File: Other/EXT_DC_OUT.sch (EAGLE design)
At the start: 19 parts, among them IC1 TINY45, Q1 IRLU3410, Q2 IRLU3410, Q3 IRLU3410, X2 PW1

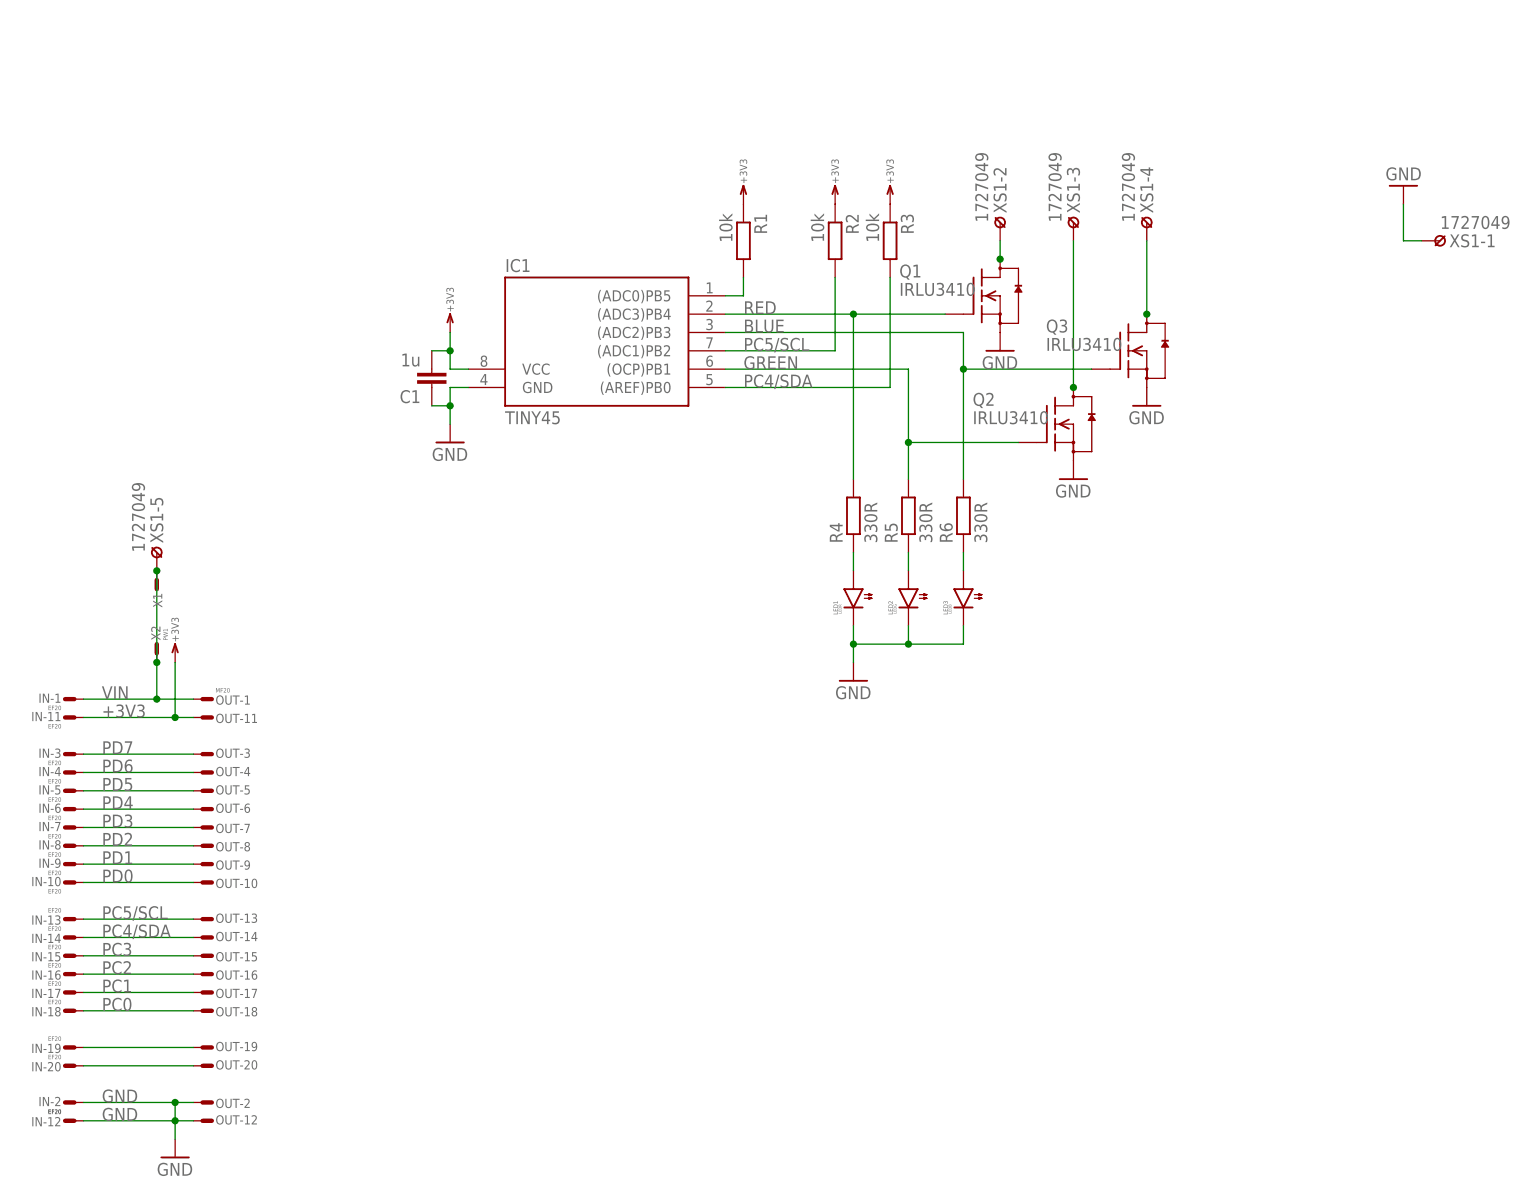
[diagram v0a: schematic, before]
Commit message: Added ...
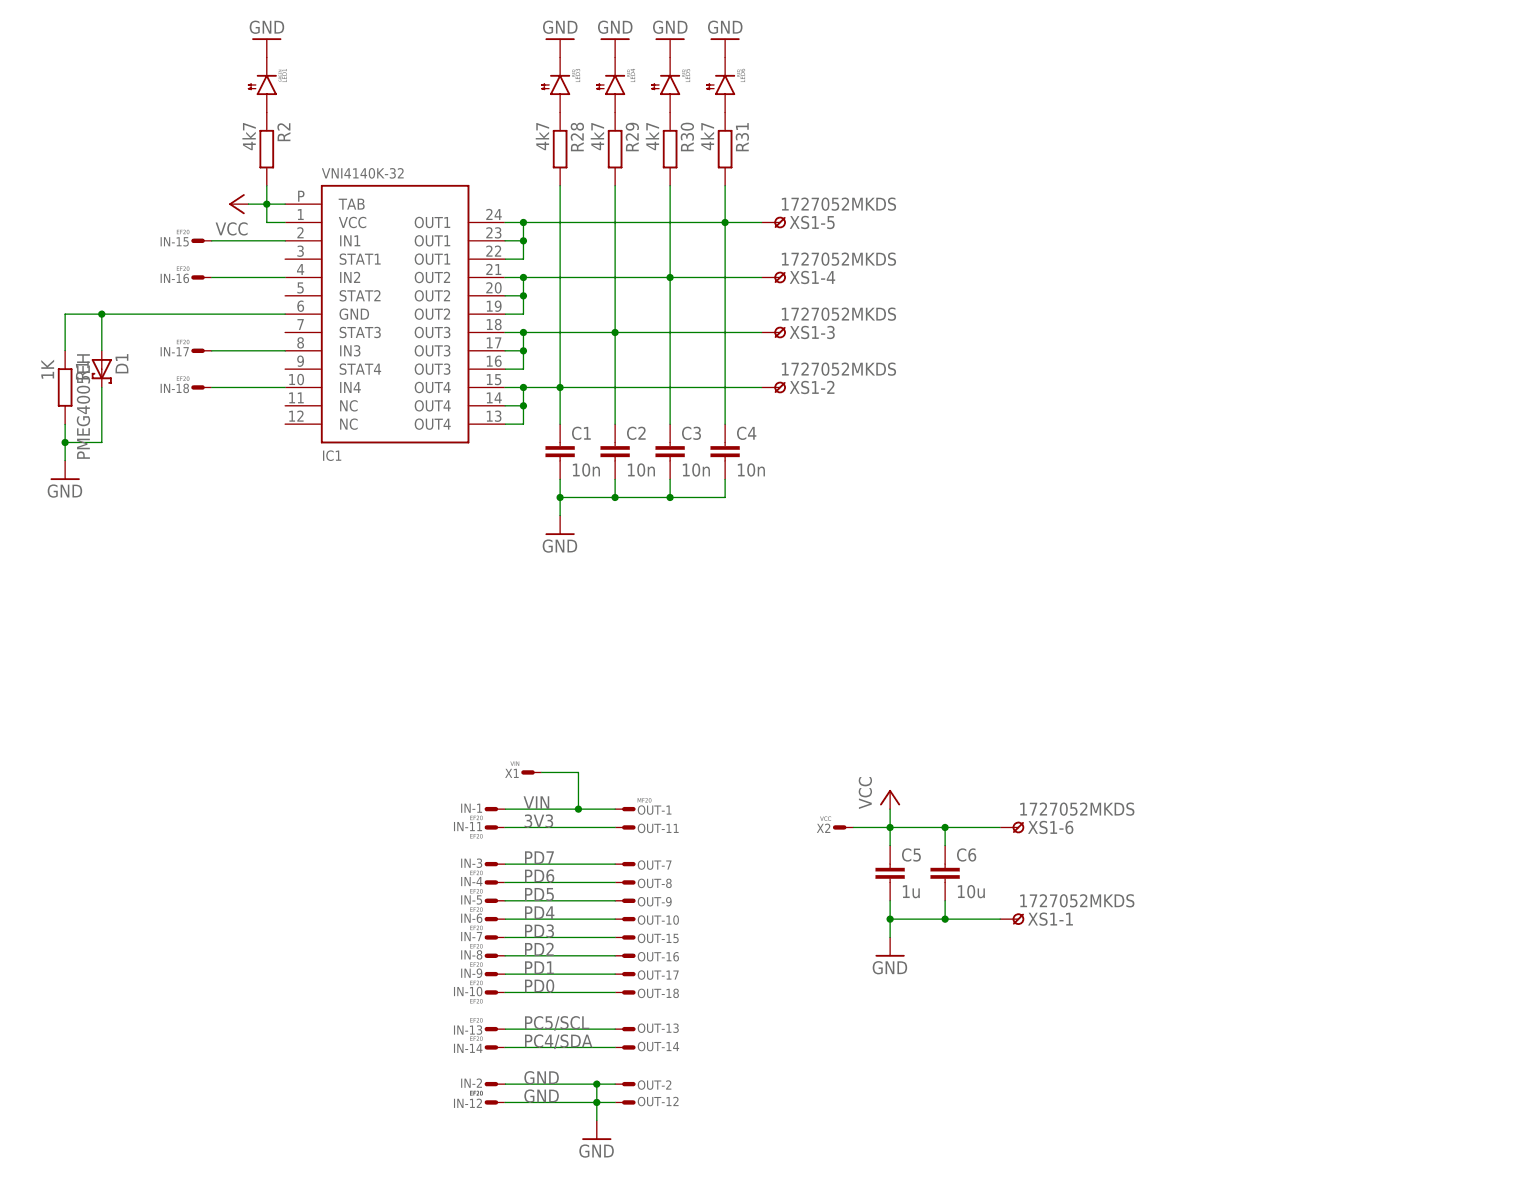
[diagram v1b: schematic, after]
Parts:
- removed LED2: LEDG, Optic:LED1206
- removed Q1, Q2, Q3: IRLU3410, Transistor:FET-ND251
- removed R3: 10k, RCL:R0603
- removed R4, R5, R6: 330R, RCL:R0603
- added C2, C3, C4: 10n, RCL:C1206
- added C5: 1u, RCL:C1206
- added C6: 10u, RCL:CC1210
- added D1: PMEG4005EH, Diode:D-SCHOTKY123
- added LED4, LED5, LED6: RED, Optic:LED1206
- added R28, R29, R30, R31: 4k7, RCL:R1206
- C1: value 1u -> 10n; device RCL:C0603 -> RCL:C1206
- IC1: value TINY45 -> VNI4140K-32; device atmel:TINY15LS -> ICs:VNI4140
- LED1: value LEDR -> GREEN
- LED3: value LEDB -> RED
- R1: value 10k -> 1K; device RCL:R0603 -> RCL:R1206
- R2: value 10k -> 4k7; device RCL:R0603 -> RCL:R1206
- X1: value (none) -> VIN
- X2: value PW1 -> VCC
- XS1: value 1727049 -> 1727052MKDS; device Conn:1727049 -> Conn:1727052MKDS
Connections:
- removed net +3V3: C1.2, IC1.VCC, IN-11.S, OUT-11.S, R1.1, R2.1, R3.1
- removed net BLUE: IC1.(ADC2)PB3, Q3.G, R6.2
- removed net GREEN: IC1.(OCP)PB1, Q2.G, R5.2
- removed net PC0: IN-18.S, OUT-18.S
- removed net PC1: IN-17.S, OUT-17.S
- removed net PC2: IN-16.S, OUT-16.S
- removed net PC3: IN-15.S, OUT-15.S
- removed net RED: IC1.(ADC3)PB4, Q1.G, R4.2
- removed net RST: IC1.(ADC0)PB5, R1.2
- new net 3V3: IN-11.S, OUT-11.S
- new net N$10: LED1.A, R2.1
- new net N$12: LED3.A, R28.1
- new net N$14: LED4.A, R29.1
- new net N$16: LED5.A, R30.1
- new net N$18: LED6.A, R31.1
- new net N$2: IC1.IN2, IN-16.S
- new net VCC: C5.1, C6.1, IC1.TAB, IC1.VCC, R2.2, X2.S, XS1-6.K
- net GND: now also C1.2, C2.2, C3.2, C4.2, C5.2, C6.2, D1.C, LED4.C, LED5.C, LED6.C, R1.2; no longer C1.1, IC1.GND, LED2.C, Q1.S, Q2.S, Q3.S
- net N$1: now also IC1.IN1, IN-15.S; no longer IN-20.S, OUT-20.S
- net N$3: now also IC1.IN3, IN-17.S; no longer IN-19.S, OUT-19.S
- net N$4: now also IC1.IN4, IN-18.S; no longer LED1.A, R4.1
- net N$5: now also C4.1, IC1.OUT1@22, IC1.OUT1@23, IC1.OUT1@24, R31.2, XS1-5.K; no longer LED2.A, R5.1
- net N$6: now also C3.1, IC1.OUT2@19, IC1.OUT2@20, IC1.OUT2@21, R30.2, XS1-4.K; no longer Q1.D, XS1-2.K
- net N$7: now also C2.1, IC1.OUT3@16, IC1.OUT3@17, IC1.OUT3@18, R29.2; no longer Q2.D
- net N$8: now also C1.1, IC1.OUT4@13, IC1.OUT4@14, IC1.OUT4@15, R28.2, XS1-2.K; no longer Q3.D, XS1-4.K
- net N$9: now also D1.A, IC1.GND, R1.1; no longer LED3.A, R6.1
- net PC4/SDA: no longer IC1.(AREF)PB0, R3.2
- net PC5/SCL: no longer IC1.(ADC1)PB2, R2.2
- net PD0: now also OUT-18.S; no longer OUT-10.S
- net PD1: now also OUT-17.S; no longer OUT-9.S
- net PD2: now also OUT-16.S; no longer OUT-8.S
- net PD3: now also OUT-15.S; no longer OUT-7.S
- net PD4: now also OUT-10.S; no longer OUT-6.S
- net PD5: now also OUT-9.S; no longer OUT-5.S
- net PD6: now also OUT-8.S; no longer OUT-4.S
- net PD7: now also OUT-7.S; no longer OUT-3.S
- net VIN: no longer X2.S, XS1-5.K
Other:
- moved on the sheet: C1, IN-1, IN-10, IN-11, IN-12, IN-13, IN-14, IN-15, IN-16, IN-17, IN-18, IN-2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
